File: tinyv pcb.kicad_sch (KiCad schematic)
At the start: 99 parts, among them J1 JST SH, J2 Pico EZmate, J5 Conn_01x09_Socket, J6 Conn_01x09_Socket, Q1 2N7002, SW1 RST, U1 MCP1700x-330xxTT, U3 STM32F072C8Tx

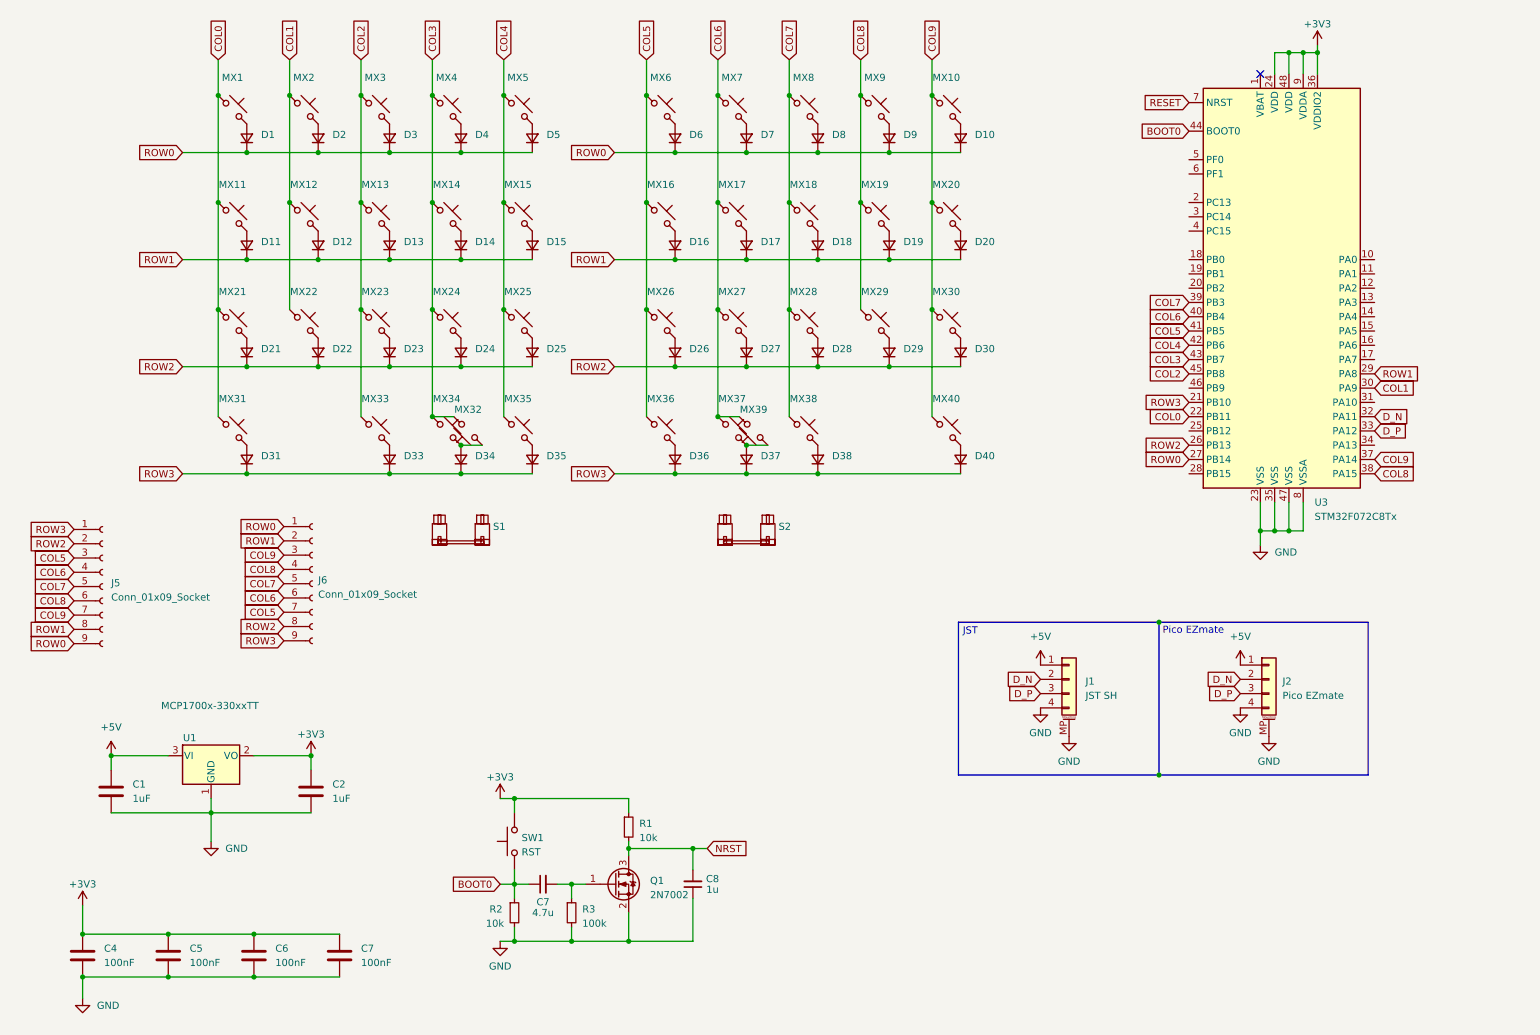
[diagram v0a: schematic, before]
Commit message: production files & bom, pos missing
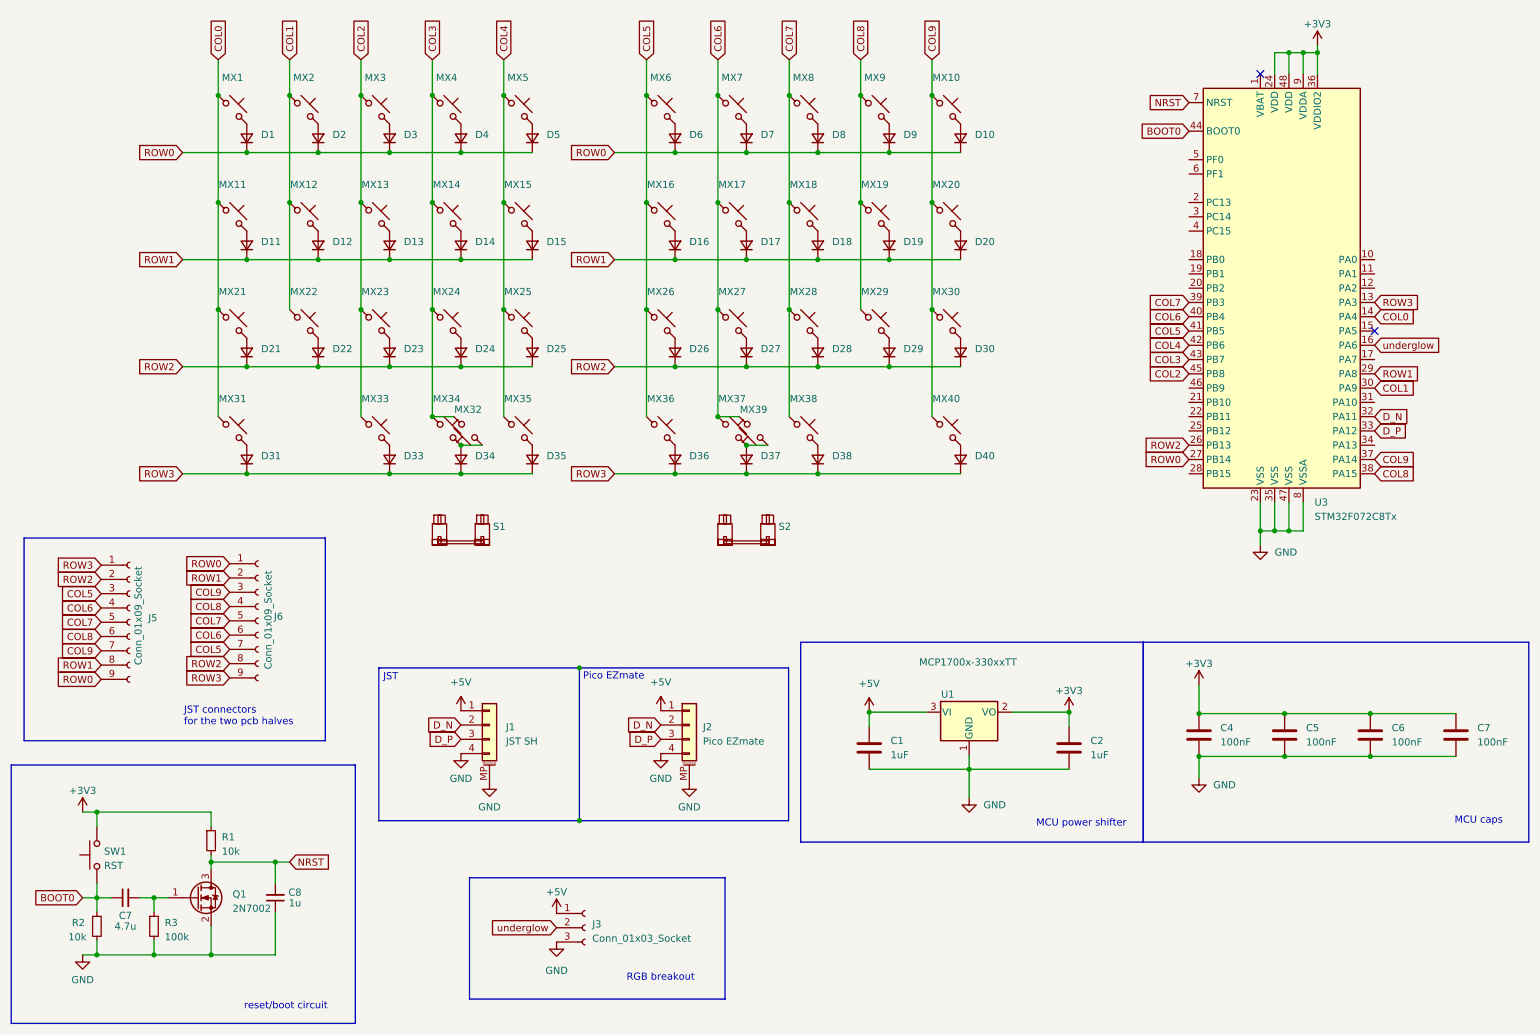
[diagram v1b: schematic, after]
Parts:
- added J3: Conn_01x03_Socket, Connector_PinHeader_2.54mm:PinHeader_1x03_P2.54mm_Vertical, symbol Connector:Conn_01x03_Socket
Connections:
- net RESET is gone; now on net NRST: U3.7 (NRST)
- net +5V: now also J3.1 (Pin_1)
- net COL0: now also U3.14 (PA4); no longer U3.22 (PB11)
- net GND: now also J3.3 (Pin_3)
- net ROW3: now also U3.13 (PA3); no longer U3.21 (PB10)
- net underglow: now reaches U3.16 (PA6)
- net underglow: now also J3.2 (Pin_2)
- no-connect marks 1 -> 2
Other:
- note added: "JST connectors for the two pcb halves"
- note added: "MCU caps"
- note added: "MCU power shifter"
- note added: "RGB breakout"
- note added: "reset/boot circuit"
- moved on the sheet: C1, C2, C4, C5, C6, C7, C8, J1, J2, J5, J6, Q1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

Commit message: slight routing change, necessary?
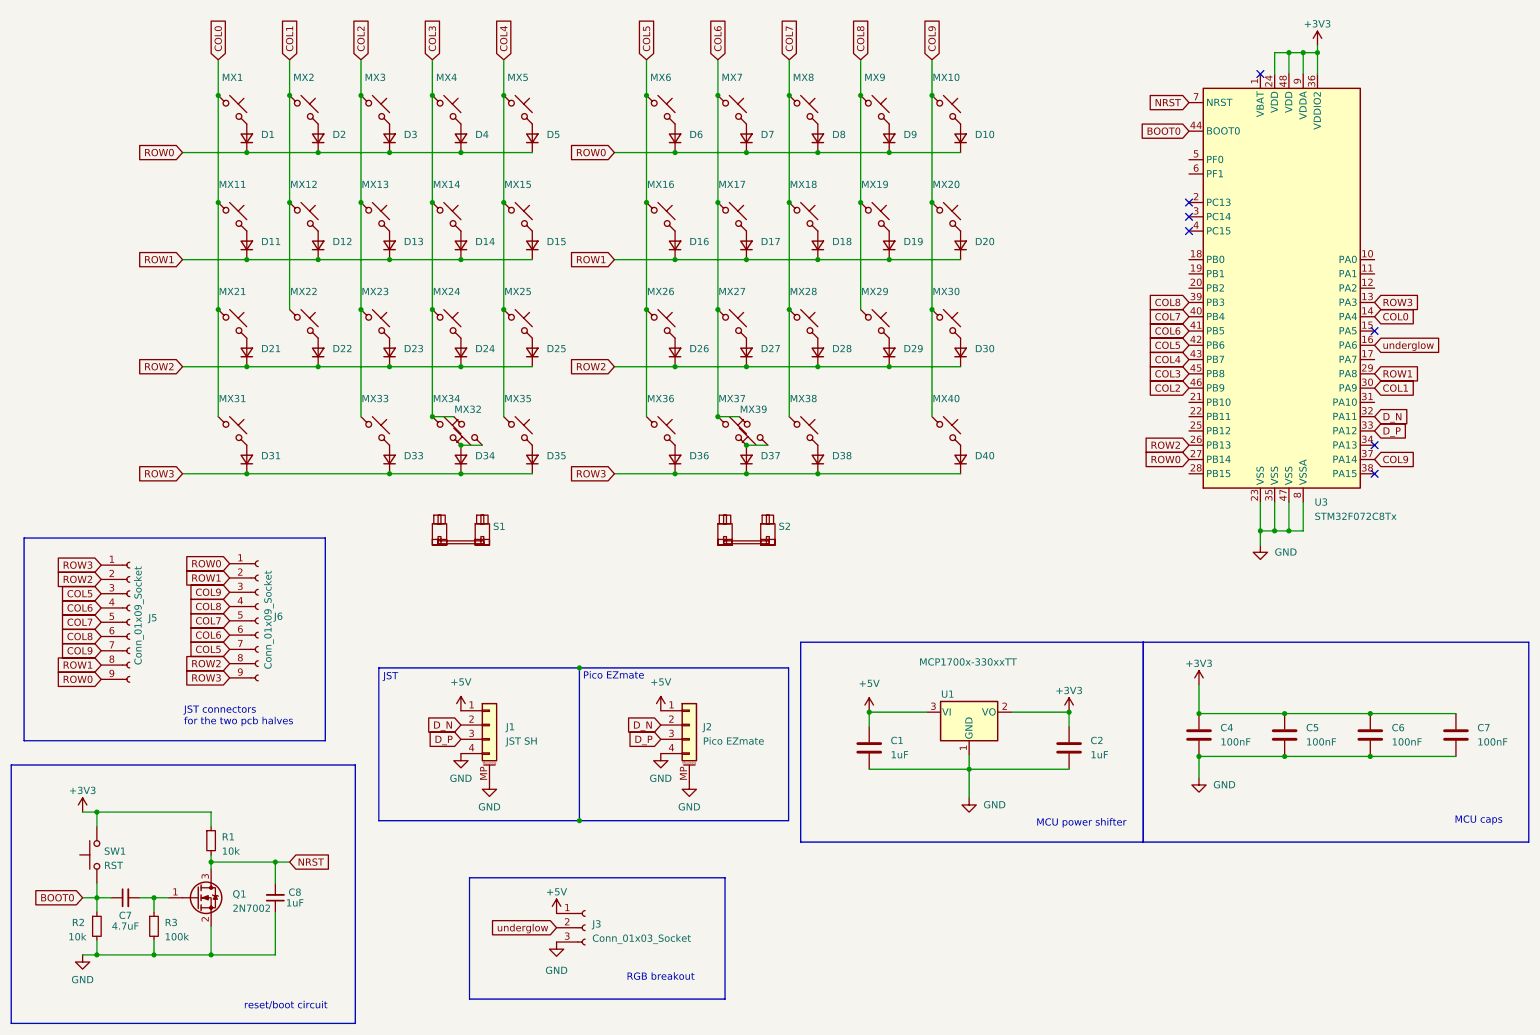
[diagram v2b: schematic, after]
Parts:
- C7: value 4.7u -> 4.7uF
- C8: value 1u -> 1uF
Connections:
- net COL2: now also U3.46 (PB9); no longer U3.45 (PB8)
- net COL3: now also U3.45 (PB8); no longer U3.43 (PB7)
- net COL4: now also U3.43 (PB7); no longer U3.42 (PB6)
- net COL5: now also U3.42 (PB6); no longer U3.41 (PB5)
- net COL6: now also U3.41 (PB5); no longer U3.40 (PB4)
- net COL7: now also U3.40 (PB4); no longer U3.39 (PB3)
- net COL8: now also U3.39 (PB3); no longer U3.38 (PA15)
- no-connect marks 2 -> 7
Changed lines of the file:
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@@
   (junction (at 39.37 174.498) (diameter 0) (color 0 0 0 0)
   )
+  (no_connect (at 223.52 55.88))
+  (no_connect (at 256.54 99.06))
+  (no_connect (at 223.52 50.8))
+  (no_connect (at 256.54 93.98))
+  (no_connect (at 223.52 53.34))
   (no_connect (at 236.22 27.94))
   (no_connect (at 256.54 73.66))
@@
     )
   )
-  (global_label "COL2" (shape input) (at 223.52 81.28 180) (fields_autoplaced)
+  (global_label "COL2" (shape input) (at 223.52 83.82 180) (fields_autoplaced)
     (effects (font (size 1.27 1.27)) (justify right))
-    (property "Intersheetrefs" "${INTERSHEET_REFS}" (at 215.7761 81.28 0)
+    (property "Intersheetrefs" "${INTERSHEET_REFS}" (at 215.7761 83.82 0)
       (effects (font (size 1.27 1.27)) (justify right) hide)
     )
@@
     )
   )
-  (global_label "COL5" (shape input) (at 223.52 73.66 180) (fields_autoplaced)
+  (global_label "COL5" (shape input) (at 223.52 76.2 180) (fields_autoplaced)
     (effects (font (size 1.27 1.27)) (justify right))
-    (property "Intersheetrefs" "${INTERSHEET_REFS}" (at 215.7761 73.66 0)
+    (property "Intersheetrefs" "${INTERSHEET_REFS}" (at 215.7761 76.2 0)
       (effects (font (size 1.27 1.27)) (justify right) hide)
     )
@@
     )
   )
-  (global_label "COL7" (shape input) (at 223.52 68.58 180) (fields_autoplaced)
+  (global_label "COL7" (shape input) (at 223.52 71.12 180) (fields_autoplaced)
     (effects (font (size 1.27 1.27)) (justify right))
-    (property "Intersheetrefs" "${INTERSHEET_REFS}" (at 215.7761 68.58 0)
+    (property "Intersheetrefs" "${INTERSHEET_REFS}" (at 215.7761 71.12 0)
       (effects (font (size 1.27 1.27)) (justify right) hide)
     )
@@
     )
   )
-  (global_label "COL3" (shape input) (at 223.52 78.74 180) (fields_autoplaced)
+  (global_label "COL3" (shape input) (at 223.52 81.28 180) (fields_autoplaced)
     (effects (font (size 1.27 1.27)) (justify right))
-    (property "Intersheetrefs" "${INTERSHEET_REFS}" (at 215.7761 78.74 0)
+    (property "Intersheetrefs" "${INTERSHEET_REFS}" (at 215.7761 81.28 0)
       (effects (font (size 1.27 1.27)) (justify right) hide)
     )
@@
     )
   )
-  (global_label "COL6" (shape input) (at 223.52 71.12 180) (fields_autoplaced)
+  (global_label "COL6" (shape input) (at 223.52 73.66 180) (fields_autoplaced)
     (effects (font (size 1.27 1.27)) (justify right))
-    (property "Intersheetrefs" "${INTERSHEET_REFS}" (at 215.7761 71.12 0)
+    (property "Intersheetrefs" "${INTERSHEET_REFS}" (at 215.7761 73.66 0)
       (effects (font (size 1.27 1.27)) (justify right) hide)
     )
@@
     )
   )
-  (global_label "COL4" (shape input) (at 223.52 76.2 180) (fields_autoplaced)
+  (global_label "COL4" (shape input) (at 223.52 78.74 180) (fields_autoplaced)
     (effects (font (size 1.27 1.27)) (justify right))
-    (property "Intersheetrefs" "${INTERSHEET_REFS}" (at 215.7761 76.2 0)
+    (property "Intersheetrefs" "${INTERSHEET_REFS}" (at 215.7761 78.74 0)
       (effects (font (size 1.27 1.27)) (justify right) hide)
     )
@@
     )
   )
-  (global_label "COL8" (shape input) (at 256.54 99.06 0) (fields_autoplaced)
-    (effects (font (size 1.27 1.27)) (justify left))
-    (property "Intersheetrefs" "${INTERSHEET_REFS}" (at 264.2839 99.06 0)
-      (effects (font (size 1.27 1.27)) (justify left) hide)
+  (global_label "COL8" (shape input) (at 223.52 68.58 180) (fields_autoplaced)
+    (effects (font (size 1.27 1.27)) (justify right))
+    (property "Intersheetrefs" "${INTERSHEET_REFS}" (at 215.7761 68.58 0)
+      (effects (font (size 1.27 1.27)) (justify right) hide)
     )
   )
@@
       (effects (font (size 1.27 1.27)))
     )
-    (property "Value" "1u" (at 64.4525 175.4505 0)
+    (property "Value" "1uF" (at 64.4525 175.4505 0)
       (effects (font (size 1.27 1.27)))
     )
@@
       (effects (font (size 1.27 1.27)))
     )
-    (property "Value" "4.7u" (at 34.29 179.578 90)
+    (property "Value" "4.7uF" (at 34.29 179.578 90)
       (effects (font (size 1.27 1.27)))
     )
